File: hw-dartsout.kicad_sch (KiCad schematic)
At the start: 52 parts, among them J1 Conn_01x10_Socket, J2 Conn_01x10_Socket, J3 Conn_01x02_Pin, J4 Conn_01x04_Pin, J5 Conn_01x10_Socket, J6 Conn_01x10_Socket, SW1 SW_Push, U1 ESP32-S2-SOLO, U2 NCP1117-3.3_SOT223

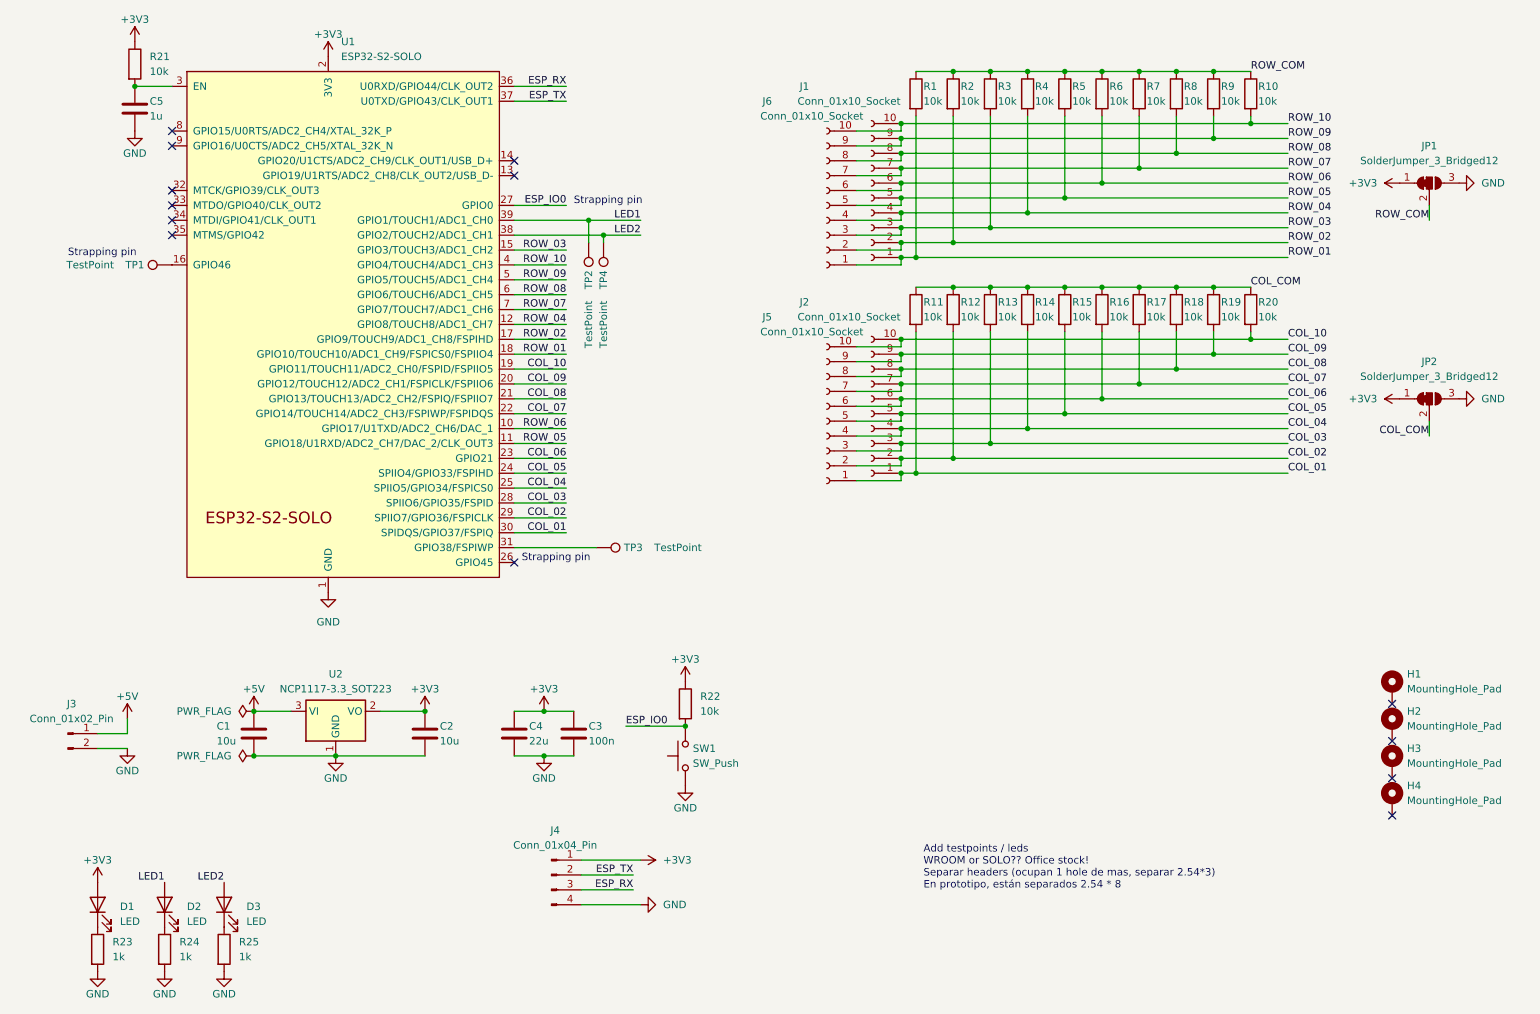
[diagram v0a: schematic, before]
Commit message: Revision 0.1
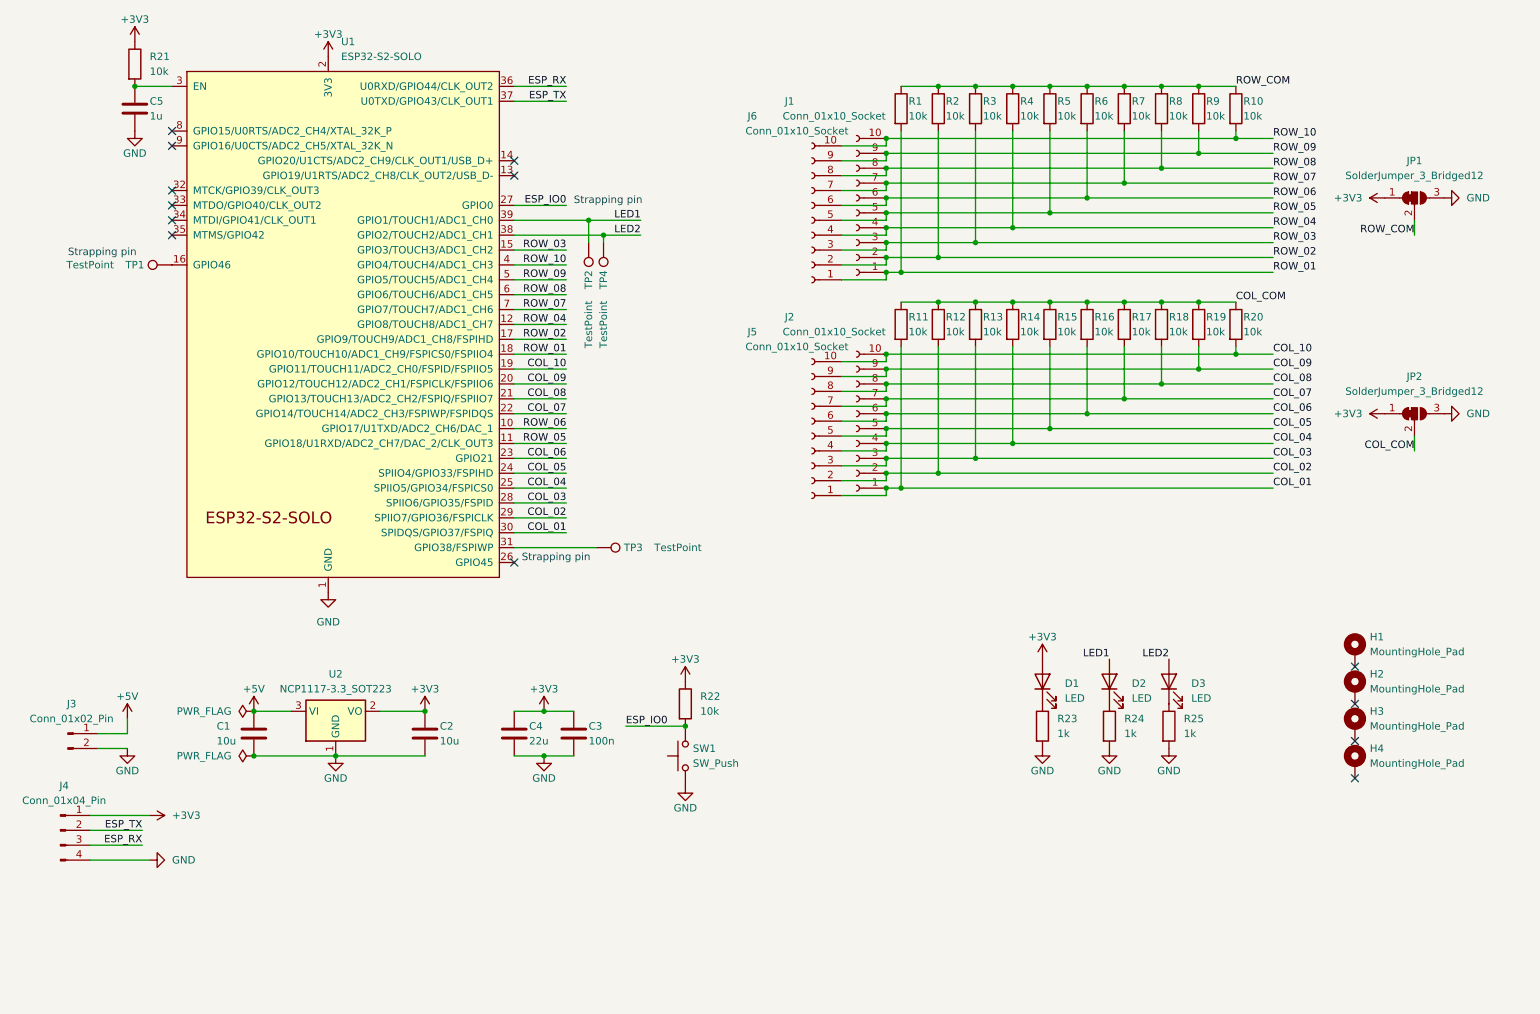
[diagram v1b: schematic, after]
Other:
- note removed: "Add testpoints / leds WROOM or SOLO?? Office stock! Separar headers (ocupan 1 hole de mas, separar 2.54*3) En prototipo, están separados 2.54 * 8"
- company: (none) -> Guille González
- title: (none) -> Dartsout
- moved on the sheet: D1, D2, D3, H1, H2, H3, H4, J1, J2, J4, J5, J6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
